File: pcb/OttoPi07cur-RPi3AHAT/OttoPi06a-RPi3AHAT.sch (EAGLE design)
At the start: 36 parts

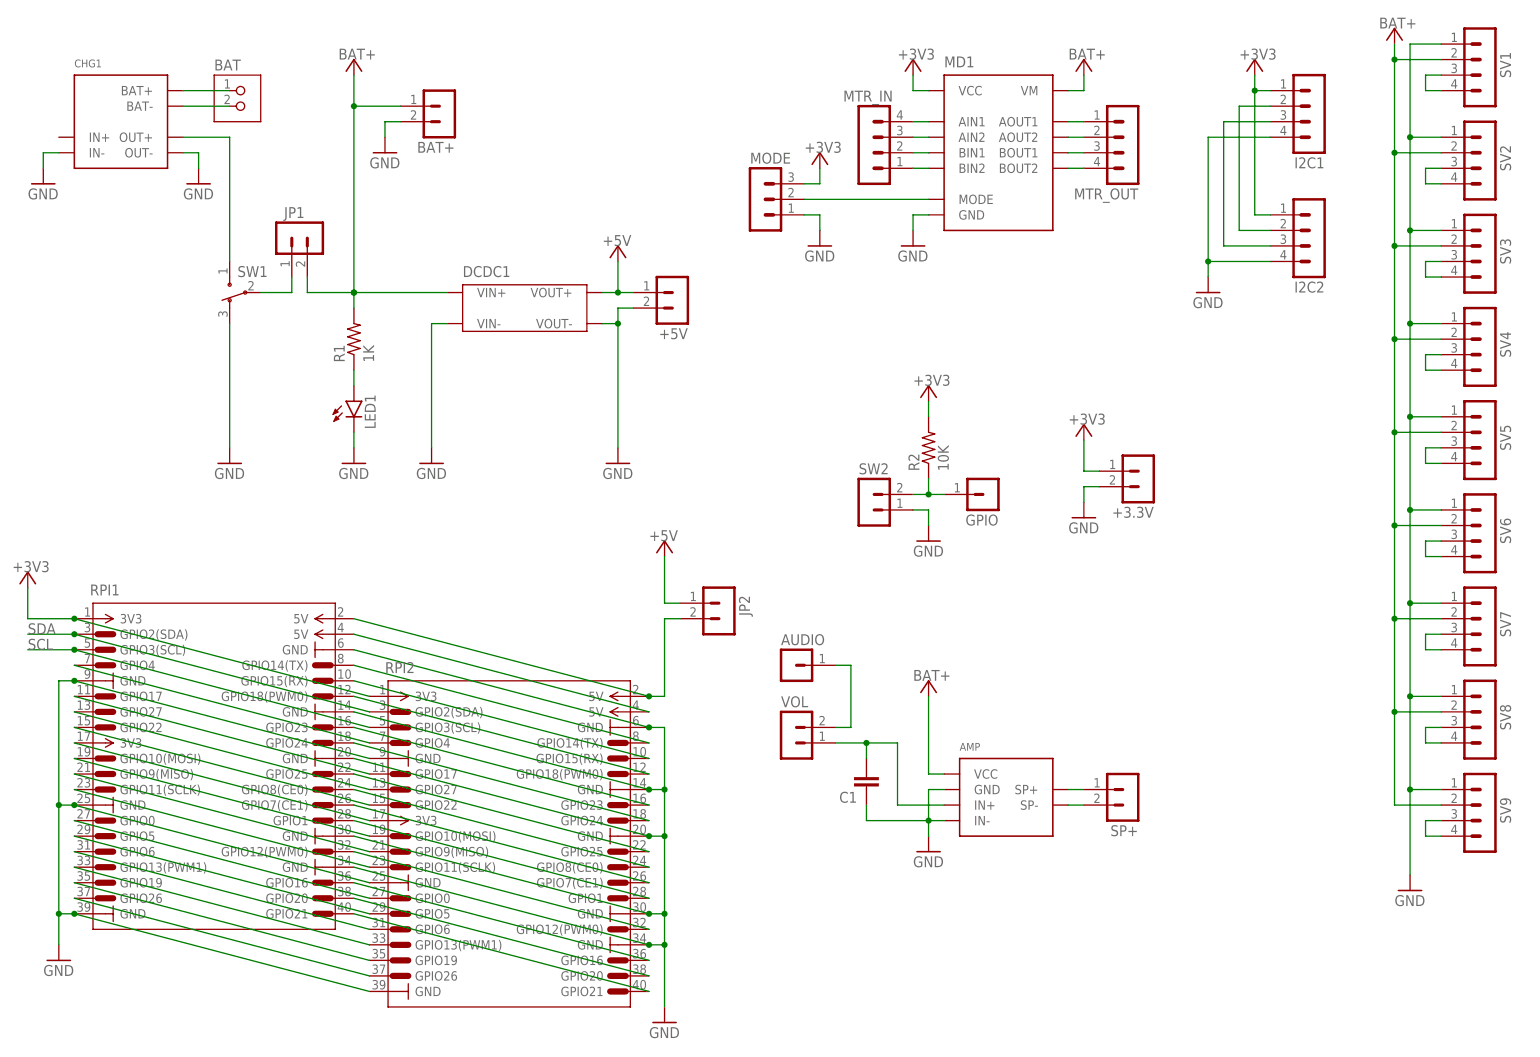
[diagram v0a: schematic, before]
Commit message: [update] PCB
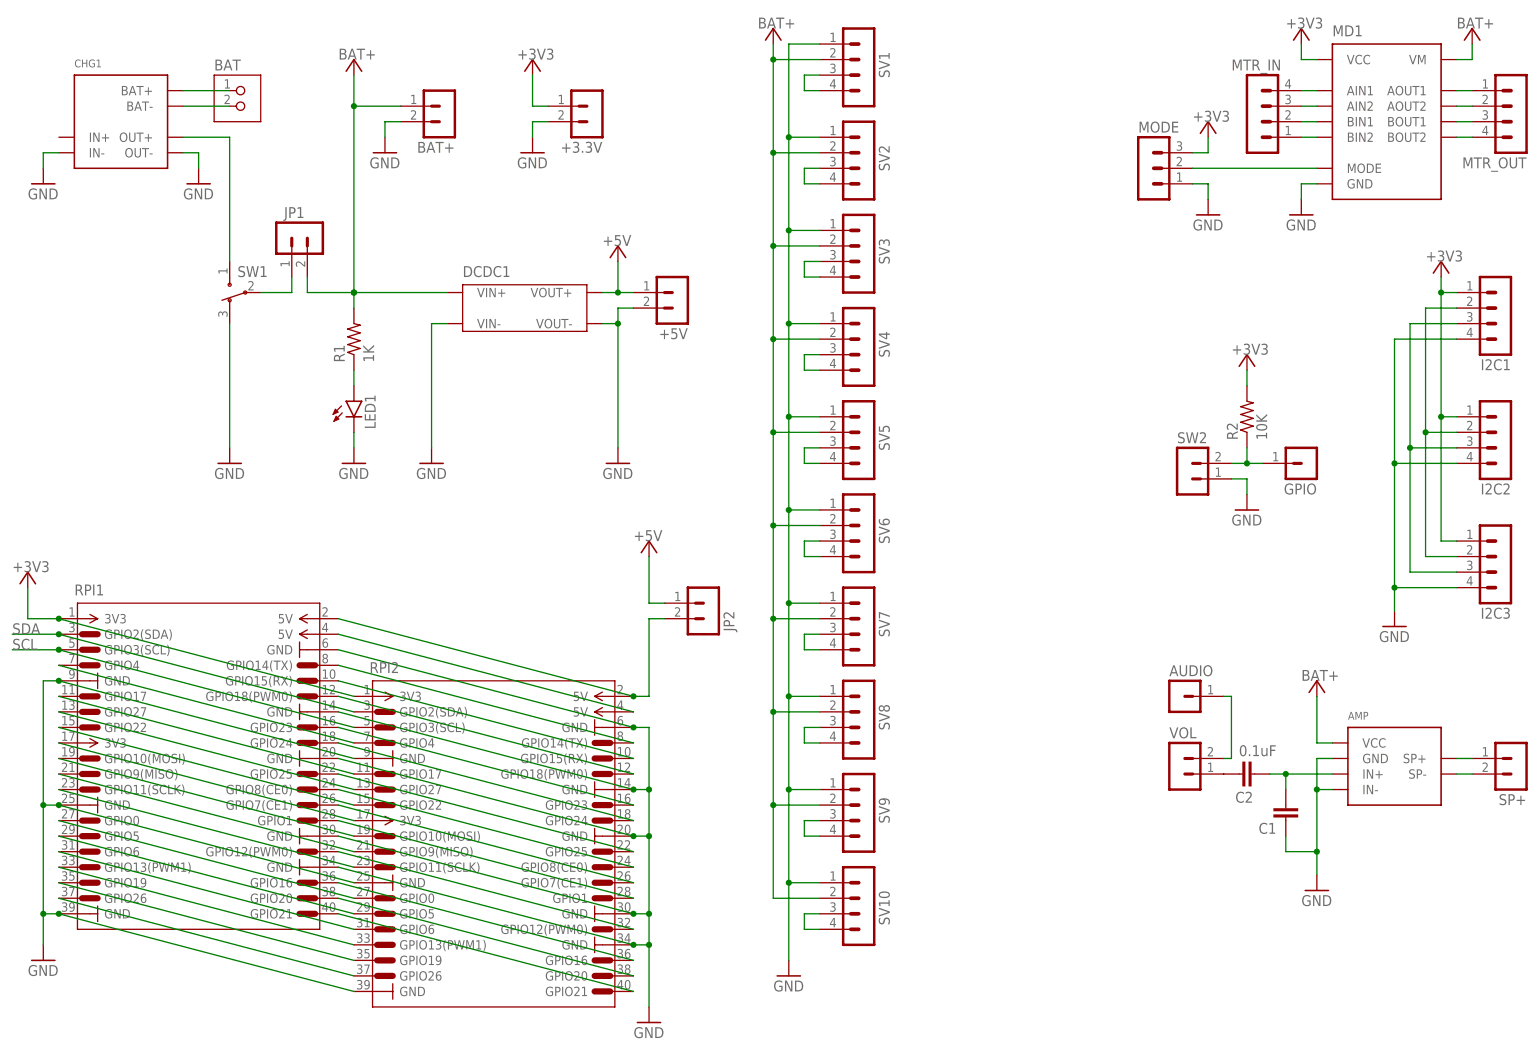
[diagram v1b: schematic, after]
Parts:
- added C2: 0.1uF, rcl:C-EU025-024X044
- added I2C3, SV10: (no value), ytani1:PINHEAD-MA04-1
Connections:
- new net N$15: C2.2, VOL.1
- new net N$17: SV10.3, SV10.4
- net +3V3: now also I2C3.1
- net AUDIO1: now also C2.1; no longer VOL.1
- net BAT+: now also SV10.2
- net GND: now also I2C3.4, SV10.1
- net SCL: now also I2C3.3
- net SDA: now also I2C3.2
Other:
- moved on the sheet: +3.3V, AMP, AUDIO, C1, GPIO, I2C1, I2C2, JP2, MD1, MODE, MTR_IN, MTR_OUT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
